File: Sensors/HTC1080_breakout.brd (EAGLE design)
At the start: 16.8 x 13.3 mm, 4 parts

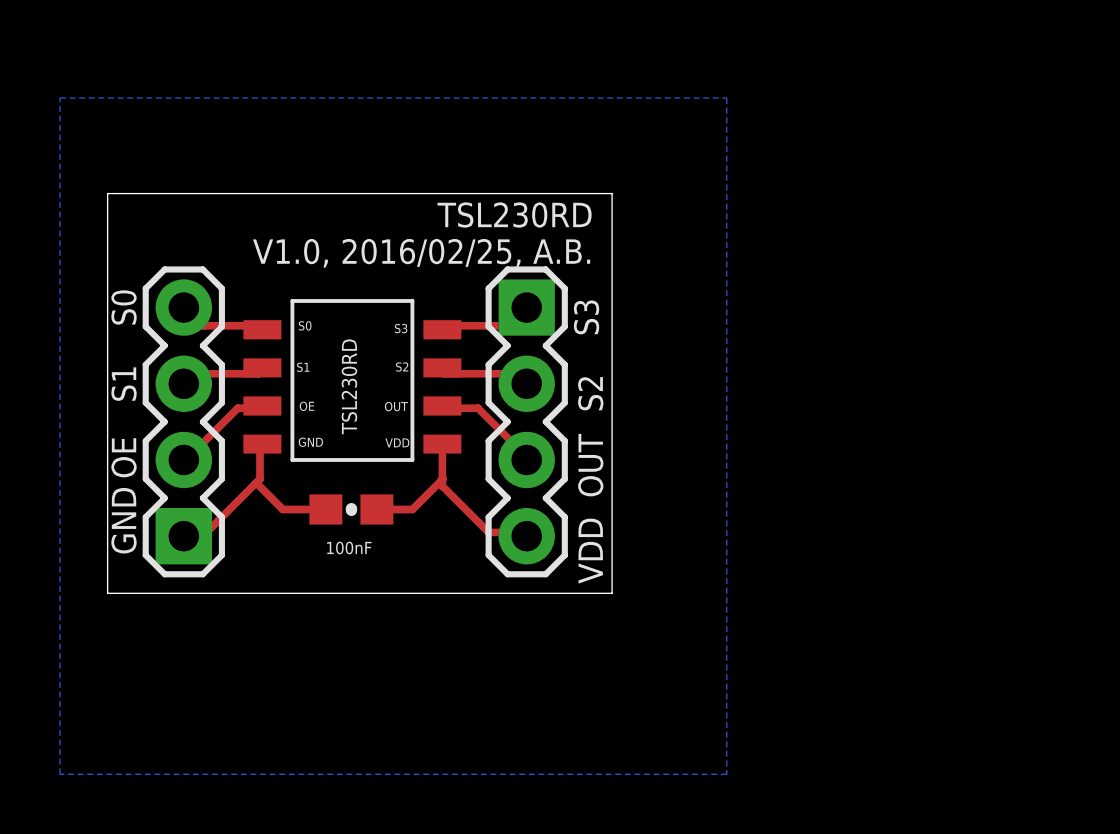
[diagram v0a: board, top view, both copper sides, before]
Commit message: new boards
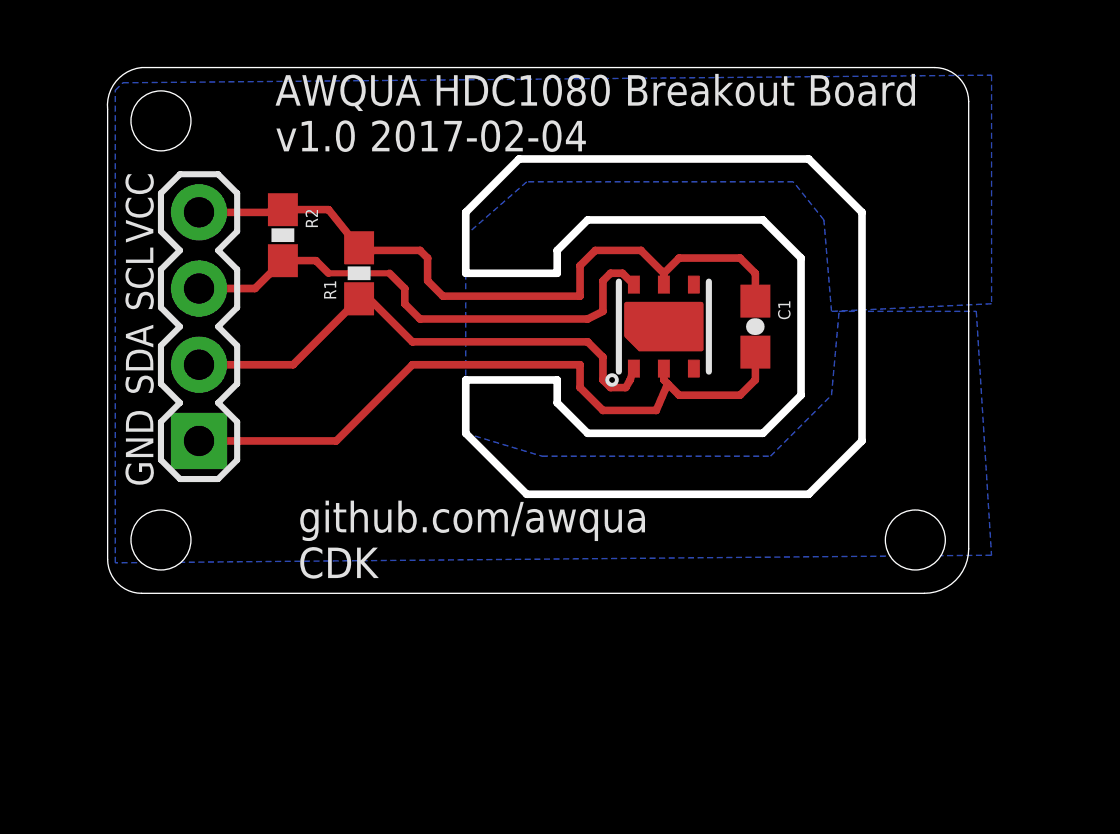
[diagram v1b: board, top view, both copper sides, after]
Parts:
- removed 100NF: 100nF, SparkFun-Capacitors:0603-CAP
- removed J1, J2: (no value), SparkFun-Connectors:1X04
- removed U$1: TSL230RDSMD, awqua_eagle_library:TSL230RD
- added C1: (no value), SparkFun-Passives:0603-CAP
- added FRAME1: FRAME-LETTER, SparkFun-Aesthetics:CREATIVE_COMMONS
- added JP1: (no value), SparkFun-Connectors:1X04
- added R1, R2: (no value), SparkFun-Passives:0603-RES
- added U1: HDC1080SMD, adam-sensors:TI-PWSON6-DMB
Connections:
- removed net N$1: J2.4, U$1.S0
- removed net N$2: J2.3, U$1.S1
- removed net N$3: J2.2, U$1.OE
- removed net N$5: J1.1, U$1.S3
- removed net N$6: J1.2, U$1.S2
- removed net N$7: J1.3, U$1.OUT
- removed net N$8: 100NF.1, J1.4, U$1.VDD
- new net SCL: JP1.3, R2.2, U1.SCL
- new net SDA: JP1.2, R1.1, U1.SDA
- new net VCC: C1.1, JP1.4, R1.2, R2.1, U1.VDD
- net GND: now also C1.2, JP1.1, U1.GND; no longer 100NF.2, J2.1, U$1.GND
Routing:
- net VCC: track 0.00 -> 23.5 mm
- net SDA: track 0.00 -> 17.5 mm
- net SCL: track 0.00 -> 17.3 mm
- net GND: track 7.22 -> 23.1 mm
- net N$8: track 7.54 -> 0.00 mm
- net N$7: track 3.62 -> 0.00 mm
- net N$3: track 3.34 -> 0.00 mm
- net N$5: track 3.22 -> 0.00 mm
- net N$6: track 3.15 -> 0.00 mm
- net N$1: track 2.91 -> 0.00 mm
- net N$2: track 2.85 -> 0.00 mm
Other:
- board size 16.8 x 13.3 mm -> 28.7 x 17.5 mm
- board text added: "AWQUA HDC1080 Breakout Board v1.0 2017-02-04"
- board text added: "Chris Kelley"
- board text added: "SCL"
- board text added: "SDA"
- board text added: "VCC"
- board text added: "github.com/awqua CDK"
- board text removed: "OE"
- board text removed: "OUT"
- board text removed: "S0"
- board text removed: "S1"
- board text removed: "S2"
- board text removed: "S3"
- board text removed: "TSL230RD V1.0, 2016/02/25, A.B."
- board text removed: "VDD"
